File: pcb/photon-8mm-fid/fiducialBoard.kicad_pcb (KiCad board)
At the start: 2 copper layers, 10 x 4 mm, 2 parts

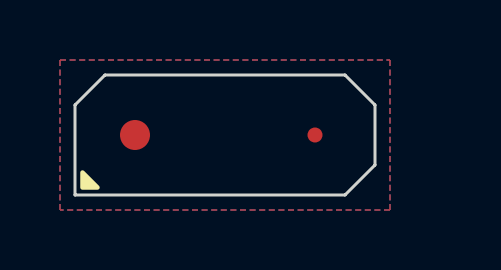
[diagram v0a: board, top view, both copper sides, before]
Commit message: pcbs and updated cad pushed up
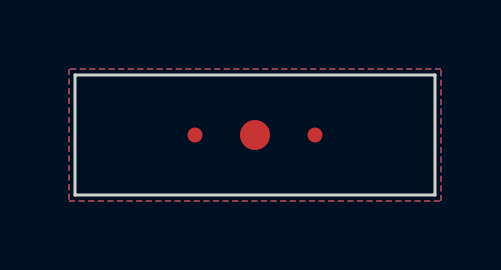
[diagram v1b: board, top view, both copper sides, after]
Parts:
- added REF**: Fiducial_0.5mm_Mask1.5mm, Fiducial:Fiducial_0.5mm_Mask1.5mm, F.Cu at (4.00, -2.00)
- moved REF** 4.00 mm to (6.00, -2.00)
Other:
- board size 10 x 4 mm -> 12 x 4 mm
- board text added: "8mm Fiducial REV01"
- board text removed: "8mm Fiducial REV00"
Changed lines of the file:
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@@
-(kicad_pcb (version 20211014) (generator pcbnew)
+(kicad_pcb (version 20221018) (generator pcbnew)
   (general
     (thickness 1)
@@
     (pcbplotparams
       (layerselection 0x00010fc_ffffffff)
+      (plot_on_all_layers_selection 0x0000000_00000000)
       (disableapertmacros false)
       (usegerberextensions false)
@@
       (usegerberadvancedattributes true)
       (creategerberjobfile true)
-      (svguseinch false)
+      (dashed_line_dash_ratio 12.000000)
+      (dashed_line_gap_ratio 3.000000)
       (svgprecision 6)
-      (excludeedgelayer true)
       (plotframeref false)
       (viasonmask false)
@@
       (drillshape 0)
       (scaleselection 1)
-      (outputdirectory "out/rev00/")
+      (outputdirectory "out/rev01/")
     )
   )
   (net 0 "")
   (footprint "Fiducial:Fiducial_1mm_Mask2mm" (layer "F.Cu")
-    (at 2 -2)
+    (at 6 -2)
     (descr "Circular Fiducial, 1mm bare copper, 2mm soldermask opening (Level A)")
     (tags "fiducial")
     (attr smd)
     (fp_text reference "REF**" (at -1 -4) (layer "F.SilkS") hide
-      (effects (font (size 1 1) (thickness 0.15)))
+        (effects (font (size 1 1) (thickness 0.15)))
     )
     (fp_text value "Fiducial_1mm_Mask2mm" (at 0 2) (layer "F.Fab")
-      (effects (font (size 1 1) (thickness 0.15)))
+        (effects (font (size 1 1) (thickness 0.15)))
     )
     (fp_text user "${REFERENCE}" (at 0 0) (layer "F.Fab")
-      (effects (font (size 0.4 0.4) (thickness 0.06)))
+        (effects (font (size 0.4 0.4) (thickness 0.06)))
     )
-    (fp_circle (center 0 0) (end 1.25 0) (layer "F.CrtYd") (width 0.05) (fill none))
-    (fp_circle (center 0 0) (end 1 0) (layer "F.Fab") (width 0.1) (fill none))
+    (fp_circle (center 0 0) (end 1.25 0)
+      (stroke (width 0.05) (type solid)) (fill none) (layer "F.CrtYd"))
+    (fp_circle (center 0 0) (end 1 0)
+      (stroke (width 0.1) (type solid)) (fill none) (layer "F.Fab"))
     (pad "" smd circle (at 0 0) (size 1 1) (layers "F.Cu" "F.Mask")
       (solder_mask_margin 0.5) (clearance 0.5))
@@
     (attr smd)
     (fp_text reference "REF**" (at 0 -4) (layer "F.SilkS") hide
-      (effects (font (size 1 1) (thickness 0.15)))
+        (effects (font (size 1 1) (thickness 0.15)))
     )
     (fp_text value "Fiducial_0.5mm_Mask1.5mm" (at 0 1.7145) (layer "F.Fab")
-      (effects (font (size 1 1) (thickness 0.15)))
+        (effects (font (size 1 1) (thickness 0.15)))
     )
     (fp_text user "${REFERENCE}" (at 0 0) (layer "F.Fab")
-      (effects (font (size 0.2 0.2) (thickness 0.04)))
+        (effects (font (size 0.2 0.2) (thickness 0.04)))
     )
-    (fp_circle (center 0 0) (end 1 0) (layer "F.CrtYd") (width 0.05) (fill none))
-    (fp_circle (center 0 0) (end 0.75 0) (layer "F.Fab") (width 0.1) (fill none))
+    (fp_circle (center 0 0) (end 1 0)
+      (stroke (width 0.05) (type solid)) (fill none) (layer "F.CrtYd"))
+    (fp_circle (center 0 0) (end 0.75 0)
+      (stroke (width 0.1) (type solid)) (fill none) (layer "F.Fab"))
     (pad "" smd circle (at 0 0) (size 0.5 0.5) (layers "F.Cu" "F.Mask")
       (solder_mask_margin 0.5) (clearance 0.5))
   )
-  (gr_poly
-    (pts
-      (xy 0.75 -0.25)
-      (xy 0.25 -0.25)
-      (xy 0.25 -0.75)
-    ) (layer "F.SilkS") (width 0.15) (fill solid))
-  (gr_line (start 0 0) (end 9 0) (layer "Edge.Cuts") (width 0.1))
-  (gr_line (start 9 0) (end 10 -1) (layer "Edge.Cuts") (width 0.1))
-  (gr_line (start 10 -3) (end 9 -4) (layer "Edge.Cuts") (width 0.1))
-  (gr_line (start 0 -3) (end 0 0) (layer "Edge.Cuts") (width 0.1))
-  (gr_line (start 9 -4) (end 1 -4) (layer "Edge.Cuts") (width 0.1))
-  (gr_line (start 10 -1) (end 10 -3) (layer "Edge.Cuts") (width 0.1))
-  (gr_line (start 0 -3) (end 1 -4) (layer "Edge.Cuts") (width 0.1))
-  (gr_text "8mm Fiducial\nREV00" (at 5 -2) (layer "B.SilkS")
+  (footprint "Fiducial:Fiducial_0.5mm_Mask1.5mm" (layer "F.Cu")
+    (at 4 -2)
+    (descr "Circular Fiducial, 0.5mm bare copper, 1.5mm soldermask opening")
+    (tags "fiducial")
+    (attr smd)
+    (fp_text reference "REF**" (at 0 -4) (layer "F.SilkS") hide
+        (effects (font (size 1 1) (thickness 0.15)))
+    )
+    (fp_text value "Fiducial_0.5mm_Mask1.5mm" (at 0 1.7145) (layer "F.Fab")
+        (effects (font (size 1 1) (thickness 0.15)))
+    )
+    (fp_text user "${REFERENCE}" (at 0 0) (layer "F.Fab")
+        (effects (font (size 0.2 0.2) (thickness 0.04)))
+    )
+    (fp_circle (center 0 0) (end 1 0)
+      (stroke (width 0.05) (type solid)) (fill none) (layer "F.CrtYd"))
+    (fp_circle (center 0 0) (end 0.75 0)
+      (stroke (width 0.1) (type solid)) (fill none) (layer "F.Fab"))
+    (pad "" smd circle (at 0 0) (size 0.5 0.5) (layers "F.Cu" "F.Mask")
+      (solder_mask_margin 0.5) (clearance 0.5))
+  )
+  (gr_line (start 0 0) (end 12 0)
+    (stroke (width 0.1) (type solid)) (layer "Edge.Cuts"))
+  (gr_line (start 0 -4) (end 0 0)
+    (stroke (width 0.1) (type solid)) (layer "Edge.Cuts"))
+  (gr_line (start 12 -4) (end 0 -4)
+    (stroke (width 0.1) (type solid)) (layer "Edge.Cuts"))
+  (gr_line (start 12 0) (end 12 -4)
+    (stroke (width 0.1) (type solid)) (layer "Edge.Cuts"))
+  (gr_text "8mm Fiducial\nREV01" (at 6 -2) (layer "B.SilkS")
     (effects (font (size 0.75 0.75) (thickness 0.1)) (justify mirror))
   )
-  (zone (net 0) (net_name "") (layers F&B.Cu) (hatch edge 0.508)
-    (connect_pads (clearance 0.508))
-    (min_thickness 0.254) (filled_areas_thickness no)
-    (fill yes (thermal_gap 0.508) (thermal_bridge_width 0.508))
+  (zone (net 0) (net_name "") (layers "F&B.Cu") (hatch edge 0.5)
+    (connect_pads (clearance 0.2))
+    (min_thickness 0.25) (filled_areas_thickness no)
+    (fill yes (thermal_gap 0.5) (thermal_bridge_width 0.5) (island_removal_mode 1) (island_area_min 10))
     (polygon
       (pts
-        (xy 10.5 0.5)
-        (xy -0.5 0.5)
-        (xy -0.5 -4.5)
-        (xy 10.5 -4.5)
+        (xy -0.2 -4.2)
+        (xy -0.2 0.2)
+        (xy 12.2 0.2)
+        (xy 12.2 -4.2)
       )
     )
